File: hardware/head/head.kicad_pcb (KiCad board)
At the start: 2 copper layers, 50.8 x 38.7 mm, 12 parts, among them J1 DB9_Male, J2 Stats_Button, J3 Flush_Button, J4 Brew_Button, J5 Temp_Ok, J6 Display, J7 HX711, J8 Rotary_Encoder, U1 Teensy4.0

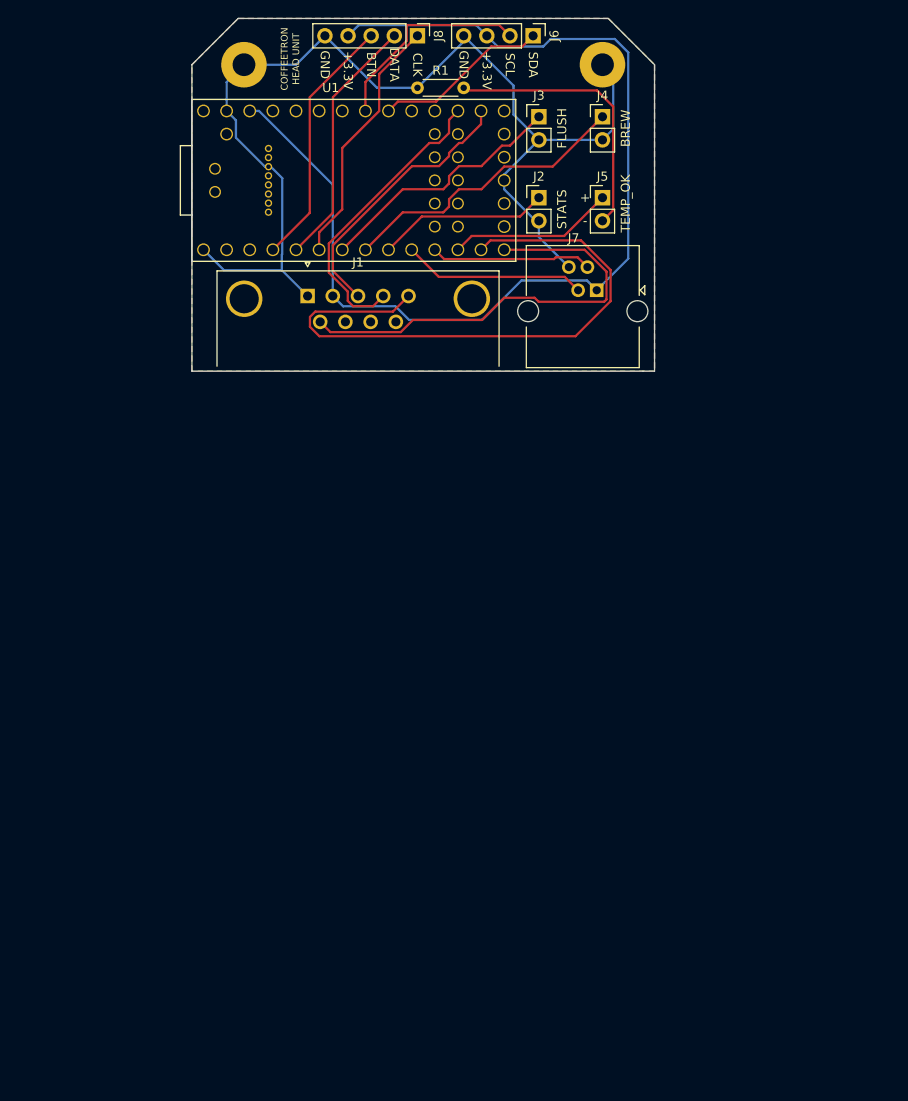
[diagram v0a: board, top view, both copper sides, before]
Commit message: Update head unit
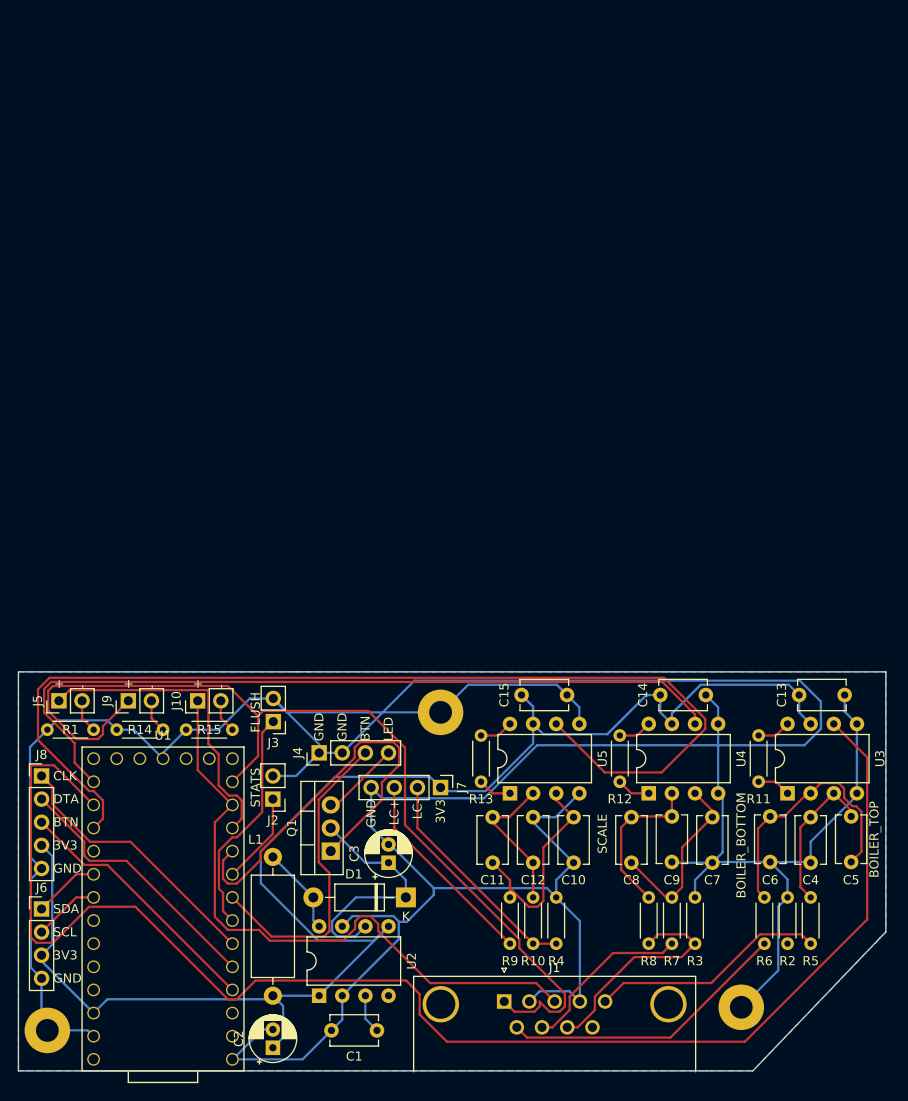
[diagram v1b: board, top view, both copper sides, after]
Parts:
- removed H1: MountingHole_Pad, MountingHole:MountingHole_2.5mm_Pad
- added C1: 0.1uF, Capacitor_THT:C_Disc_D5.1mm_W3.2mm_P5.00mm, F.Cu at (95.9, 160.7)
- added C10: 1nF, Capacitor_THT:C_Disc_D5.1mm_W3.2mm_P5.00mm, F.Cu at (117.5, 142.2)
- added C11: 10nF, Capacitor_THT:C_Disc_D5.1mm_W3.2mm_P5.00mm, F.Cu at (108.6, 142.2)
- added C12: 1nF, Capacitor_THT:C_Disc_D5.1mm_W3.2mm_P5.00mm, F.Cu at (113.0, 142.2)
- added C13: 0.1uF, Capacitor_THT:C_Disc_D5.1mm_W3.2mm_P5.00mm, F.Cu at (142.2, 123.8)
- added C14: 0.1uF, Capacitor_THT:C_Disc_D5.1mm_W3.2mm_P5.00mm, F.Cu at (127.0, 123.8)
- added C15: 0.1uF, Capacitor_THT:C_Disc_D5.1mm_W3.2mm_P5.00mm, F.Cu at (111.8, 123.8)
- added C2: 150uF, Capacitor_THT:CP_Radial_D5.0mm_P2.00mm, F.Cu at (84.5, 162.6)
- added C3: 100uF, Capacitor_THT:CP_Radial_D5.0mm_P2.00mm, F.Cu at (97.2, 142.2)
- added C4: 1nF, Capacitor_THT:C_Disc_D5.1mm_W3.2mm_P5.00mm, F.Cu at (143.5, 142.2)
- added C5: 10nF, Capacitor_THT:C_Disc_D5.1mm_W3.2mm_P5.00mm, F.Cu at (148.0, 137.2)
- added C6: 1nF, Capacitor_THT:C_Disc_D5.1mm_W3.2mm_P5.00mm, F.Cu at (139.1, 137.2)
- added C7: 1nF, Capacitor_THT:C_Disc_D5.1mm_W3.2mm_P5.00mm, F.Cu at (132.7, 142.2)
- added C8: 10nF, Capacitor_THT:C_Disc_D5.1mm_W3.2mm_P5.00mm, F.Cu at (123.8, 142.2)
- added C9: 1nF, Capacitor_THT:C_Disc_D5.1mm_W3.2mm_P5.00mm, F.Cu at (128.3, 137.2)
- added D1: 1N5817, Diode_THT:D_DO-41_SOD81_P10.16mm_Horizontal, F.Cu at (99.1, 146.1)
- added H3: MountingHole_Pad, MountingHole:MountingHole_2.5mm_Pad, F.Cu at (102.9, 125.7)
- added H4: MountingHole_Pad, MountingHole:MountingHole_2.5mm_Pad, F.Cu at (59.7, 160.7)
- added J10: Pump_Active, Connector_PinHeader_2.54mm:PinHeader_1x02_P2.54mm_Vertical, F.Cu at (76.2, 124.5)
- added J9: Heater_Active, Connector_PinHeader_2.54mm:PinHeader_1x02_P2.54mm_Vertical, F.Cu at (68.6, 124.5)
- added L1: 22uH, Inductor_THT:L_Axial_L11.0mm_D4.5mm_P15.24mm_Horizontal_Fastron_MECC, F.Cu at (84.5, 156.8)
- added Q1: IRF540N, Package_TO_SOT_THT:TO-220-3_Vertical, F.Cu at (90.8, 141.0)
- added R10: 10k, Resistor_THT:R_Axial_DIN0204_L3.6mm_D1.6mm_P5.08mm_Horizontal, F.Cu at (113.0, 151.1)
- added R11: 400, Resistor_THT:R_Axial_DIN0204_L3.6mm_D1.6mm_P5.08mm_Horizontal, F.Cu at (137.8, 133.3)
- added R12: 400, Resistor_THT:R_Axial_DIN0204_L3.6mm_D1.6mm_P5.08mm_Horizontal, F.Cu at (122.6, 133.3)
- added R13: 650, Resistor_THT:R_Axial_DIN0204_L3.6mm_D1.6mm_P5.08mm_Horizontal, F.Cu at (107.3, 133.3)
- added R14: 220, Resistor_THT:R_Axial_DIN0204_L3.6mm_D1.6mm_P5.08mm_Horizontal, F.Cu at (72.4, 127.6)
- added R15: 220, Resistor_THT:R_Axial_DIN0204_L3.6mm_D1.6mm_P5.08mm_Horizontal, F.Cu at (80.0, 127.6)
- added R2: 1M, Resistor_THT:R_Axial_DIN0204_L3.6mm_D1.6mm_P5.08mm_Horizontal, F.Cu at (141.0, 151.1)
- added R3: 1M, Resistor_THT:R_Axial_DIN0204_L3.6mm_D1.6mm_P5.08mm_Horizontal, F.Cu at (130.8, 151.1)
- added R4: 1M, Resistor_THT:R_Axial_DIN0204_L3.6mm_D1.6mm_P5.08mm_Horizontal, F.Cu at (115.6, 151.1)
- added R5: 10k, Resistor_THT:R_Axial_DIN0204_L3.6mm_D1.6mm_P5.08mm_Horizontal, F.Cu at (143.5, 151.1)
- added R6: 10k, Resistor_THT:R_Axial_DIN0204_L3.6mm_D1.6mm_P5.08mm_Horizontal, F.Cu at (138.4, 151.1)
- added R7: 10k, Resistor_THT:R_Axial_DIN0204_L3.6mm_D1.6mm_P5.08mm_Horizontal, F.Cu at (128.3, 151.1)
- added R8: 10k, Resistor_THT:R_Axial_DIN0204_L3.6mm_D1.6mm_P5.08mm_Horizontal, F.Cu at (125.7, 151.1)
- added R9: 10k, Resistor_THT:R_Axial_DIN0204_L3.6mm_D1.6mm_P5.08mm_Horizontal, F.Cu at (110.5, 151.1)
- added U2: MAX757, Package_DIP:DIP-8_W7.62mm, F.Cu at (89.5, 156.8)
- added U3: INA126, Package_DIP:DIP-8_W7.62mm, F.Cu at (141.0, 134.6)
- added U4: INA126, Package_DIP:DIP-8_W7.62mm, F.Cu at (125.7, 134.6)
- added U5: INA126, Package_DIP:DIP-8_W7.62mm, F.Cu at (110.5, 134.6)
- J4: footprint Connector_PinHeader_2.54mm:PinHeader_1x02_P2.54mm_Vertical -> Connector_PinHeader_2.54mm:PinHeader_1x04_P2.54mm_Vertical
- J7: value HX711 -> Load_Cell; footprint Connector_RJ:RJ14_Connfly_DS1133-S4_Horizontal -> Connector_PinHeader_2.54mm:PinHeader_1x04_P2.54mm_Vertical
- moved J6 110.0 mm to (59.1, 147.3), turned to 0 degrees
- moved H2 104.6 mm to (135.9, 158.1)
- moved J8 91.2 mm to (59.1, 132.7), turned to 0 degrees
- moved U1 82.7 mm to (72.4, 147.3), turned to 90 degrees
- moved R1 81.4 mm to (64.8, 127.6)
- moved J5 81.3 mm to (61.0, 124.5), turned to 90 degrees
- moved J1 80.4 mm to (109.9, 157.5)
- moved J4 76.5 mm to (89.5, 130.2), turned to 90 degrees
- moved J3 72.5 mm to (84.5, 126.7), turned to 180 degrees
- moved J2 72.2 mm to (84.5, 135.3), turned to 180 degrees
- moved J7 57.2 mm to (102.9, 134.0), turned to 270 degrees
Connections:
- J1 pad 1: GND -> HEATER_SSR+
- J1 pad 2: +3V3 -> GND
- J1 pad 3: PUMP_TEMP -> PUMP_SSR+
- J1 pad 4: GROUPHEAD_TEMP -> GND
- J1 pad 5: PUMP -> BOILER_TOP_TEMP+
- J1 pad 6: HEATER_RELAY -> BOILER_TOP_TEMP-
- J1 pad 7: Net-(J1-Pad7) -> BOILER_BOTTOM_TEMP+
- J1 pad 8: Net-(J1-Pad8) -> BOILER_BOTTOM_TEMP-
- J4 pad 1: BREW_BUTTON -> GND
- J7 pad 2: HX711_SCK -> LOAD_CELL-
- J7 pad 3: HX711_DT -> LOAD_CELL+
- U1 pad 10: HX711_DT -> BREW_READY
- U1 pad 11: HX711_SCK -> TEMP_OK
- U1 pad 12: TEMP_OK -> PUMP_SSR+
- U1 pad 13: PUMP -> HEATER_SSR+
- U1 pad 14: HEATER_RELAY -> Net-(U1-Pad14)
- U1 pad 21: PUMP_TEMP -> BOILER_BOTTOM_TEMP
- U1 pad 22: GROUPHEAD_TEMP -> BOILER_TOP_TEMP
- U1 pad 23: Net-(U1-Pad23) -> SCALE_OUT
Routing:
- net GND: track 120.1 -> 431.3 mm
- net BOILER_TOP_TEMP: track 0.00 -> 159.0 mm
- net SCALE_OUT: track 0.00 -> 116.2 mm
- net HEATER_SSR+: track 0.00 -> 109.9 mm
- net BOILER_BOTTOM_TEMP: track 0.00 -> 86.8 mm
- net PUMP_SSR+: track 0.00 -> 70.4 mm
- net PUMP: track 67.3 -> 0.00 mm
- net +3V3: track 117.7 -> 168.0 mm
- net HEATER_RELAY: track 49.0 -> 0.00 mm
- net BREW_READY: track 0.00 -> 45.4 mm
- net GROUPHEAD_TEMP: track 32.8 -> 0.00 mm
- net BOILER_TOP_TEMP-: track 0.00 -> 31.9 mm
- net PUMP_TEMP: track 30.1 -> 0.00 mm
- net Net-(C5-Pad2): track 0.00 -> 29.2 mm
- net +5V: track 0.00 -> 27.2 mm
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- removed copper zone on F.Cu, net GND
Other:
- board size 50.8 x 38.7 mm -> 95.2 x 43.8 mm
- board text added: "3V3"
- board text added: "BOILER_BOTTOM"
- board text added: "BOILER_TOP"
- board text added: "DTA"
- board text added: "LC+"
- board text added: "LC-"
- board text added: "LED"
- board text added: "SCALE"
- board text removed: "+3.3V"
- board text removed: "BREW"
- board text removed: "COFFEETRON"
- board text removed: "DATA"
- board text removed: "HEAD UNIT"
- board text removed: "TEMP_OK"

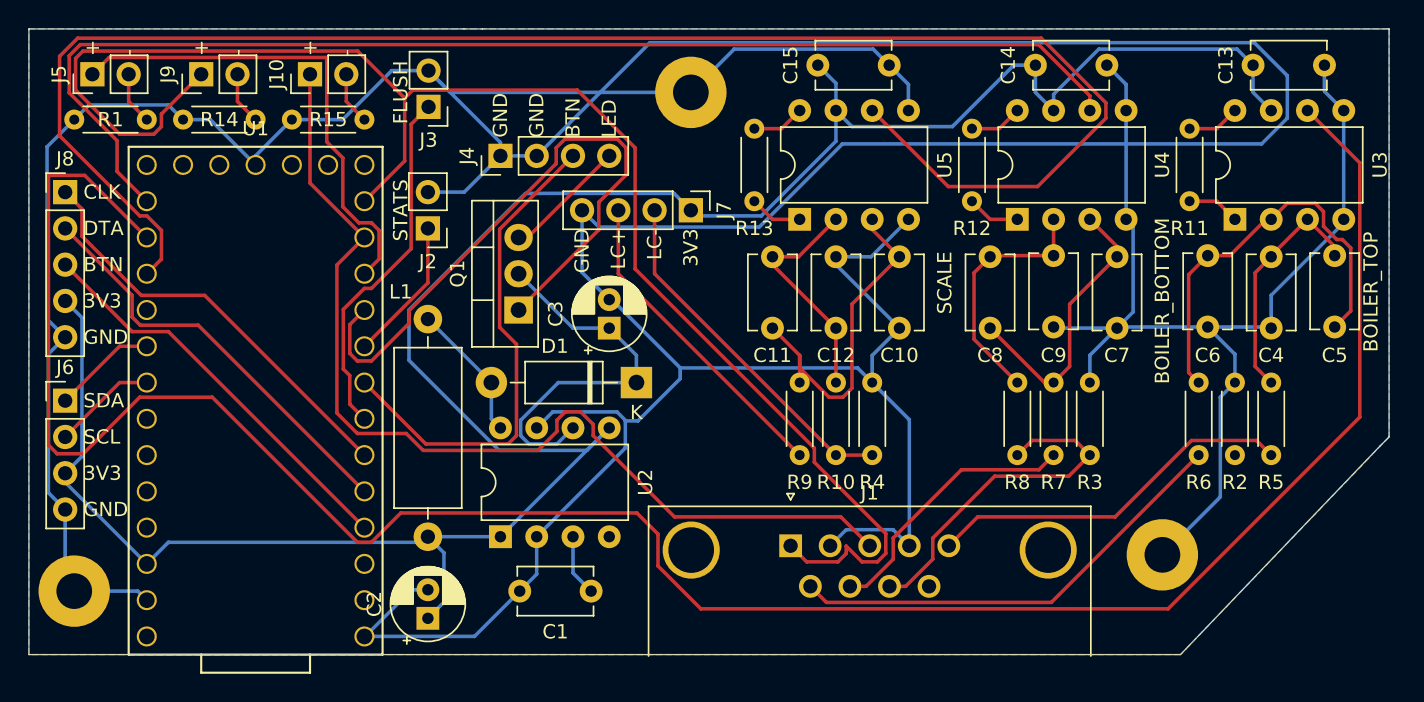
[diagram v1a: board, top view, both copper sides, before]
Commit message: Move inductor
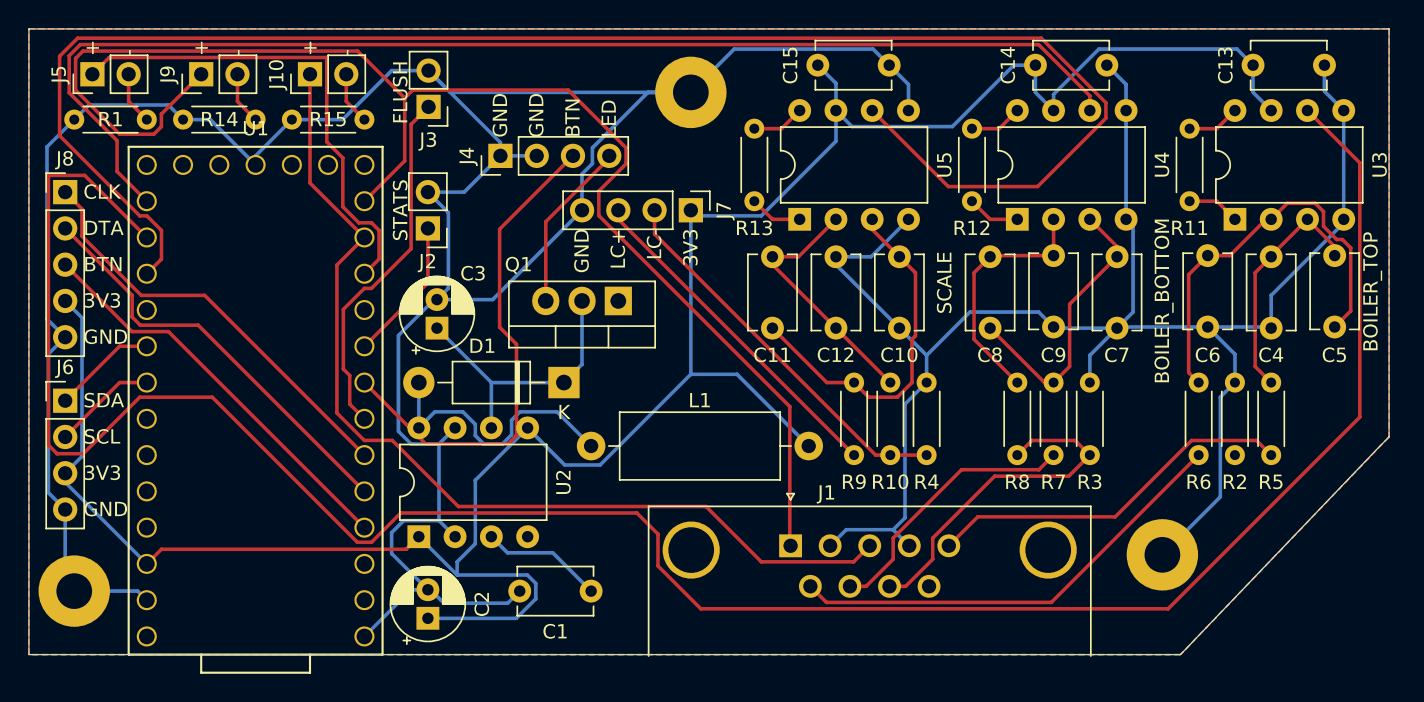
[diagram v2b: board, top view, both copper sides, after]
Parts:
- moved L1 27.4 mm to (111.1, 150.5), turned to 180 degrees
- moved C3 12.1 mm to (85.1, 142.2)
- moved Q1 7.01 mm to (97.8, 140.3), turned to 180 degrees
- moved U2 5.72 mm to (83.8, 156.8)
- moved D1 5.08 mm to (94.0, 146.1)
- moved R10 3.81 mm to (116.8, 151.1)
- moved R4 3.81 mm to (119.4, 151.1)
- moved R9 3.81 mm to (114.3, 151.1)
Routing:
- net GND: track 431.3 -> 332.3 mm
- net BREW_READY: track 45.4 -> 0.00 mm
- net HEATER_SSR+: track 109.9 -> 99.2 mm
- net Net-(D1-Pad2): track 9.72 -> 19.6 mm
- net +5V: track 27.2 -> 19.9 mm
- net Net-(C1-Pad1): track 4.34 -> 8.56 mm
- net Net-(J4-Pad4): track 8.72 -> 12.0 mm
- net PUMP_SSR+: track 70.4 -> 68.2 mm
- net LOAD_CELL-: track 24.9 -> 27.1 mm
- net Net-(C11-Pad2): track 16.2 -> 17.8 mm
- net LOAD_CELL+: track 22.4 -> 24.0 mm
- net Net-(C10-Pad2): track 24.2 -> 25.0 mm
- added copper zone on F.Cu, net GND
